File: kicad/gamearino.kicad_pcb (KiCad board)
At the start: 2 copper layers, 60 x 56 mm, 60 parts, among them Q1 PMBT3904,215, Q2 PMBT3904,215, SW1 Left, SW2 Up, SW3 Down, SW4 Right, SW5 Select, SW6 Start, SW7 B, SW8 A, U1 ESP-12F, U2 CH340C, U3 AMS1117-3.3, U4 QG-2864KSWEG01, X1 USB-C/16p

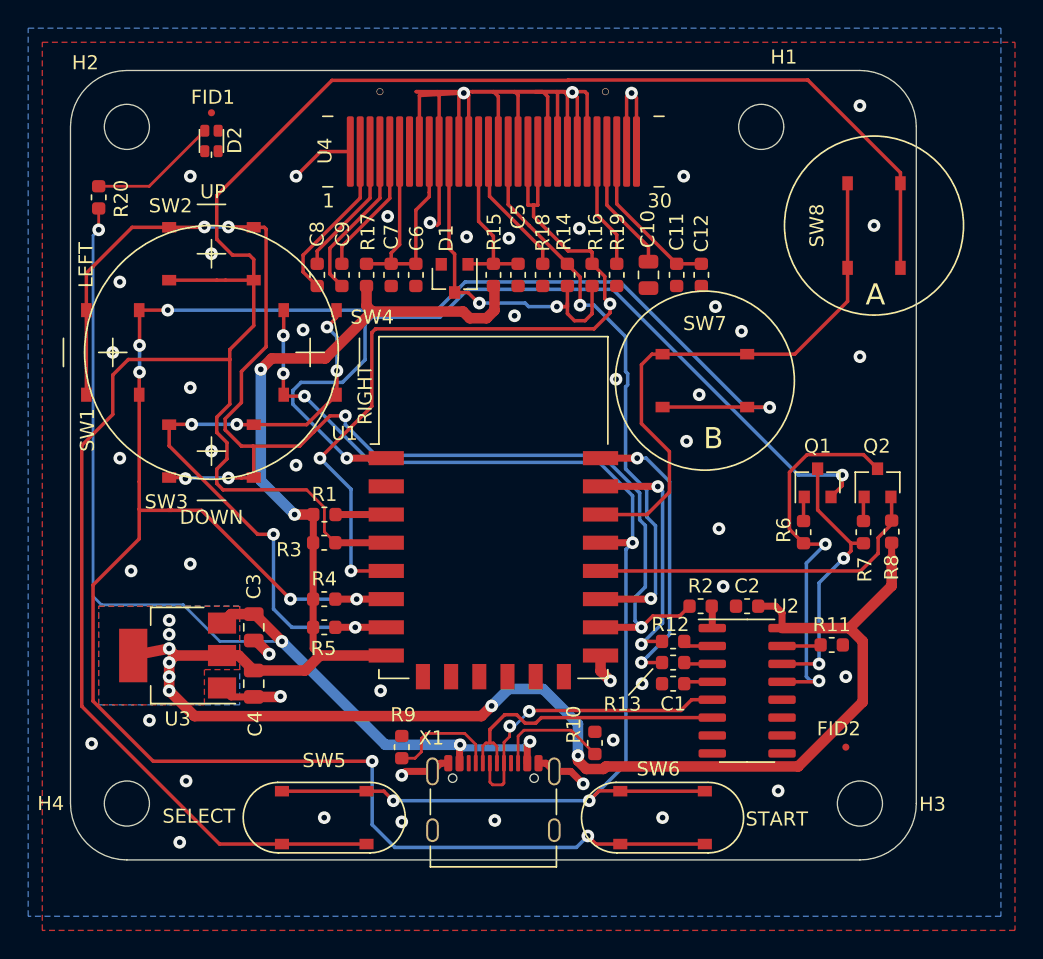
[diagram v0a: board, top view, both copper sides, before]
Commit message: wip
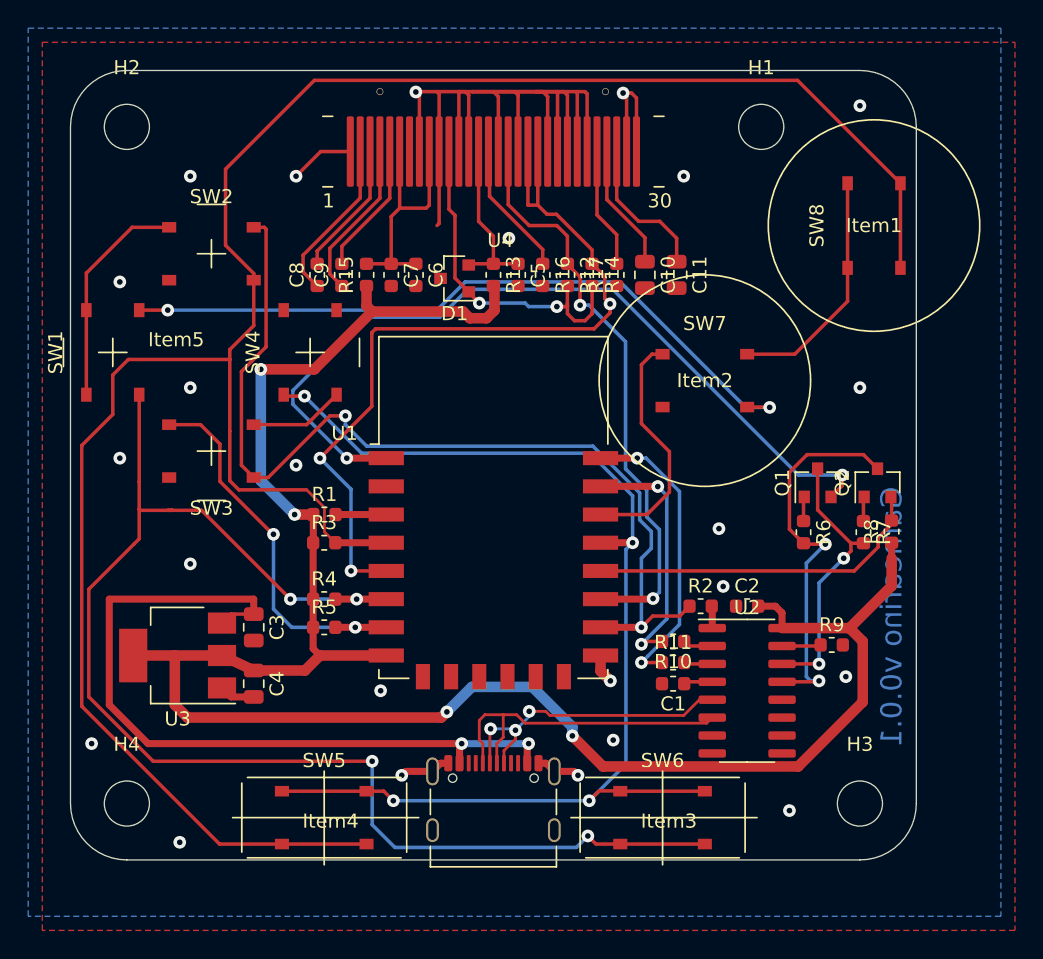
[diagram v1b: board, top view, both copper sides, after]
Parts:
- removed C12: 1u, Capacitor_SMD:C_0603_1608Metric
- removed D2: LED_Dual_green-red, htl_smd:LED_LiteOn_LTST-C195KGJRKT
- removed FID1, FID2: Fiducial, htl_mechanical:paste-fiducial
- removed the R10 at (137.2, 91.7)
- removed R20: 4k7, Resistor_SMD:R_0603_1608Metric
- removed the R9 at (123.5, 92.0)
- C10: value 10u/16V/X5R -> 4u7
- C11: value 1u -> 2u2; footprint Capacitor_SMD:C_0603_1608Metric -> Capacitor_SMD:C_0805_2012Metric
- D1: value BAV99 -> 1N4148
- Item1, Item2: footprint gamearino:ABKnopf_v2 -> gamearino:ABKnopf
- Item3, Item4: footprint gamearino:StartSelect_v2 -> gamearino:StartSelect
- Item5: footprint gamearino:Steuerkreuz_zeik_v2 -> gamearino:Steuerkreuz_zeik
- moved C10 0.25 mm to (140.8, 58.5)
- turned D1 to 180 degrees
- renumbered X1 to J1, R12 to R10, R13 to R11, R14 to R12, R15 to R13, R16 to R14, R17 to R15, R18 to R16, R19 to R17, R11 to R9
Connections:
- net /EN renamed Net-(R1-Pad2)
- D1 pad 1: Net-(C5-Pad1) -> Net-(D1-Pad1)
- D1 pad 2: (no net) -> Net-(C5-Pad1)
- D1 pad 3: Net-(D1-Pad3) -> (no net)
- J1 pad A5: Net-(R9-Pad2) -> (no net)
- J1 pad B5: Net-(R10-Pad1) (its old number) -> (no net)
- R12 pad 2: Net-(D1-Pad3) -> Net-(D1-Pad1)
- R14 pad 2: Net-(D1-Pad3) -> Net-(D1-Pad1)
- U2 pad 10: GND -> (no net)
- U2 pad 11: GND -> (no net)
- U2 pad 12: GND -> (no net)
- U2 pad 9: GND -> (no net)
- U4 pad 11: Net-(D1-Pad3) -> Net-(D1-Pad1)
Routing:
- net Net-(D1-Pad3): track 25.4 -> 0.00 mm, vias 2 -> 0
- net Net-(D1-Pad1): track 0.00 -> 24.8 mm, vias 0 -> 2
- net Net-(C3-Pad1): track 71.6 -> 55.1 mm, vias 4 -> 2
- net /Buttons/C0: track 97.1 -> 84.4 mm, vias 6 -> 2
- net /Buttons/R2: track 46.1 -> 34.2 mm, vias 6 -> 2
- net /Buttons/R1: track 158.9 -> 147.1 mm, vias 8 -> 6
- net GND: track 109.2 -> 99.1 mm, vias 50 -> 24
- net Net-(D2-Pad2): track 9.16 -> 0.00 mm
- net /Buttons/R0: track 163.5 -> 154.5 mm
- net Net-(R10-Pad1) (its old number): track 8.25 -> 0.00 mm
- net Net-(R9-Pad2): track 8.19 -> 0.00 mm
- net /Buttons/C1: track 89.5 -> 83.5 mm, vias 6 -> 4
- net /Buttons/C2: track 40.3 -> 34.3 mm
- net /USB/D-: track 21.2 -> 23.9 mm
- net Net-(C6-Pad1): track 20.1 -> 17.7 mm
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- removed copper zone on B.Cu, net +3V3
- removed copper zone on F.Cu, net +3V3
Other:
- net class Default: clearance 0.15 -> 0.25; trace_width 0.15 -> 0.25
- rule trace_clearance: 0.15 -> 0.25
- rule trace_min: 0.15 -> 0.2
- board text added: "Gamearino v0.0.1"
- board text removed: "A"
- board text removed: "AMS1117-3.3"
- board text removed: "B"
- board text removed: "CH340C"
- board text removed: "DOWN"
- board text removed: "ESP-12F (ESP8266) Arduino IDE settings compatible with NodeMCU V1.0"
- board text removed: "Gamearino V0.0.2"
- board text removed: "HTL STEYR 2021"
- board text removed: "LEFT"
- board text removed: "RIGHT"
- board text removed: "SELECT"
- board text removed: "START"
- board text removed: "UP"
- board text removed: "V0.0.2"
- board text removed: "github.com/KarlZeilhofer/gamearino"
